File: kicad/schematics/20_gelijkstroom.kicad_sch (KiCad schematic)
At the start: 8 parts

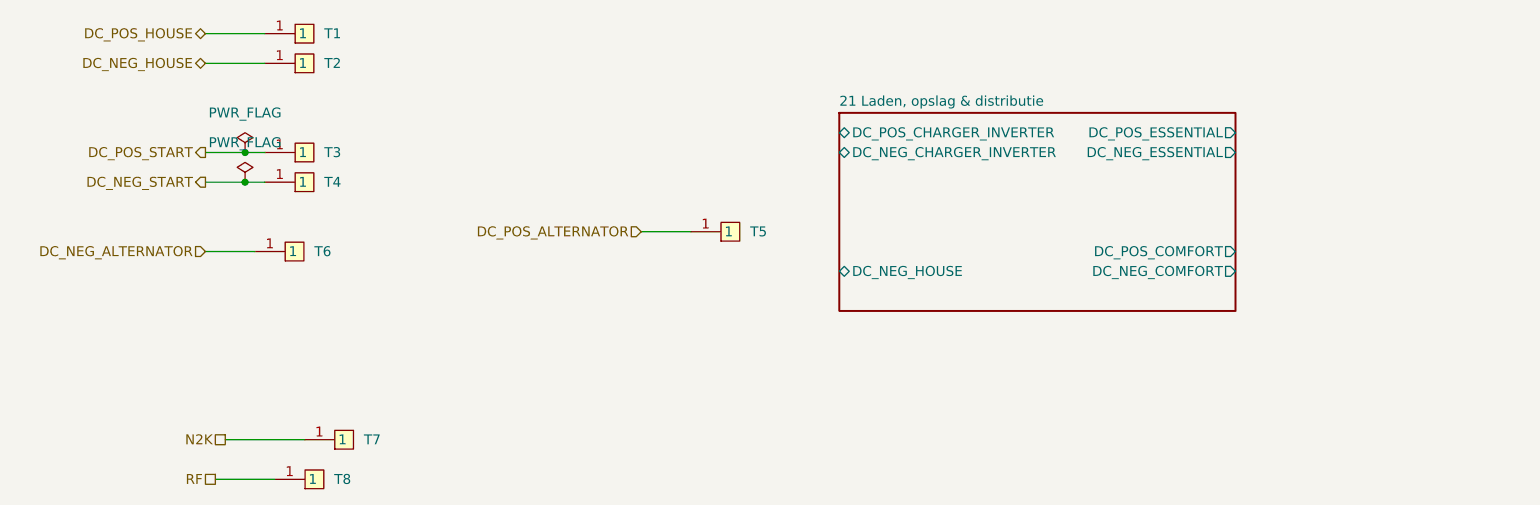
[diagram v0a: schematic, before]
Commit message: Vervolg 21_laden_opslag_distributie
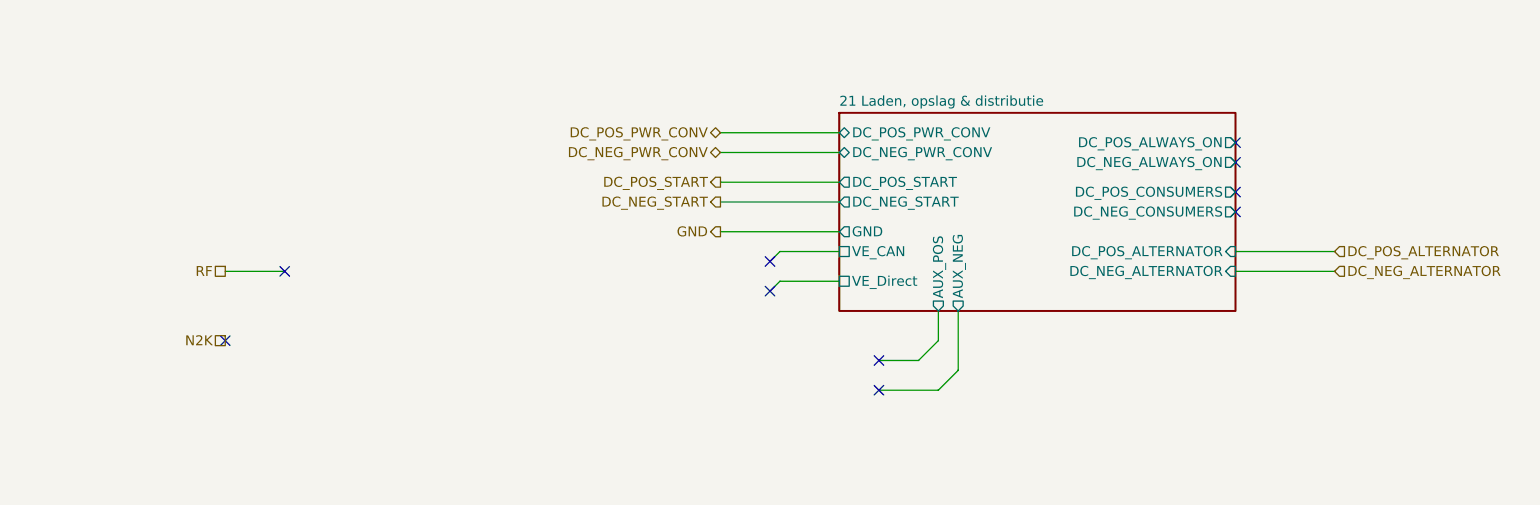
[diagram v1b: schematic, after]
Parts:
- removed T1, T2, T7, T8: (no value), symbol falkor-electrical:IF_Passief
- removed T3, T4, T5, T6: (no value), symbol falkor-electrical:IF_Power_Input
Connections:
- no-connect marks 0 -> 10
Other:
- sheet 21 Laden, opslag & distributie ports: added AUX_NEG, AUX_POS, DC_NEG_ALTERNATOR, DC_NEG_ALWAYS_ON, DC_NEG_CONSUMERS, DC_NEG_PWR_CONV, DC_NEG_START, DC_POS_ALTERNATOR, DC_POS_ALWAYS_ON, DC_POS_CONSUMERS, DC_POS_PWR_CONV, DC_POS_START, GND, VE_CAN, VE_Direct; removed DC_NEG_CHARGER_INVERTER, DC_NEG_COMFORT, DC_NEG_ESSENTIAL, DC_NEG_HOUSE, DC_POS_CHARGER_INVERTER, DC_POS_COMFORT, DC_POS_ESSENTIAL
